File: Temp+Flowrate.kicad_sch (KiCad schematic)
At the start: 24 parts, among them Q1 IRLML0030TRPBF, Q2 IRLML0030TRPBF, U2 TLV9002QDRQ1

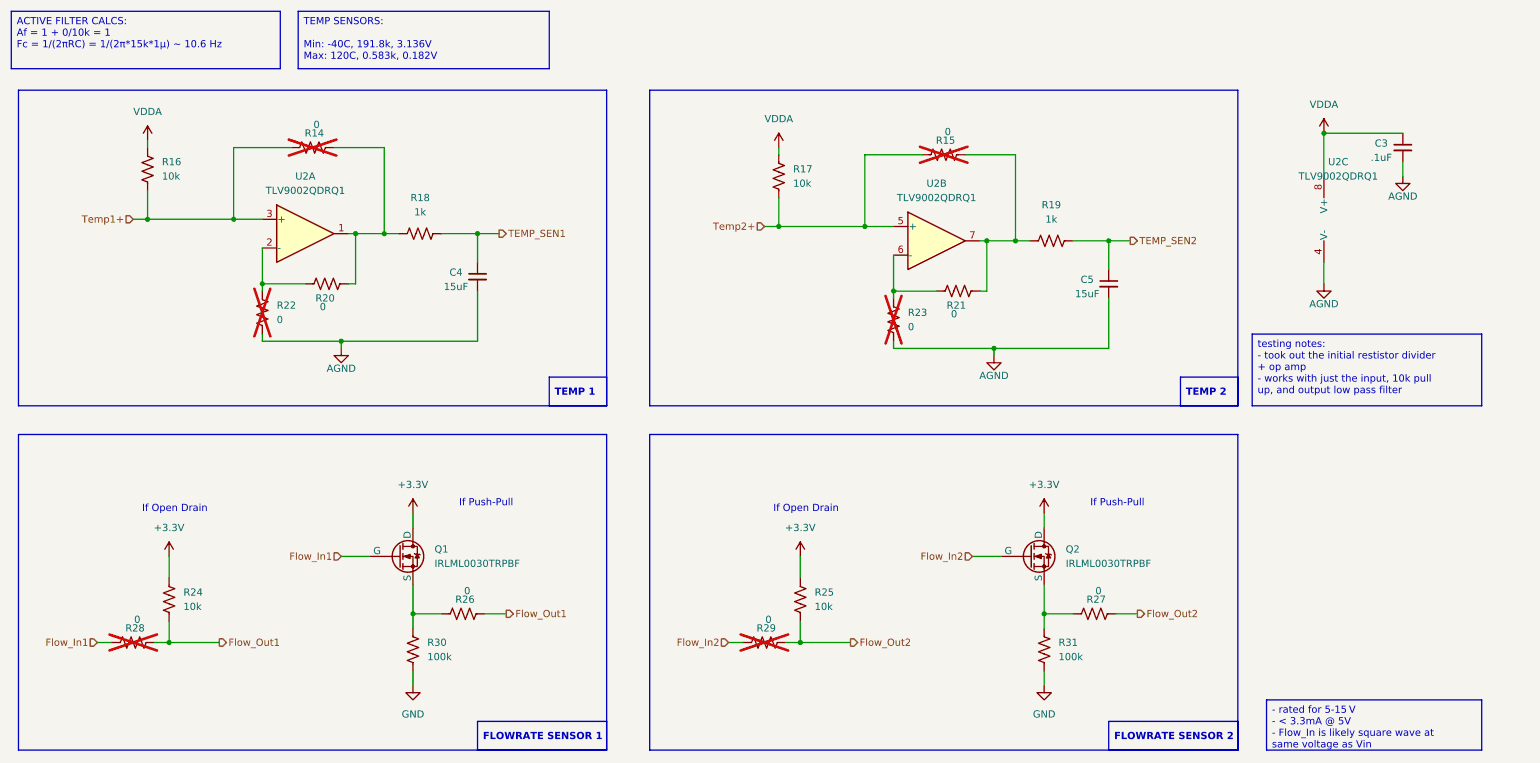
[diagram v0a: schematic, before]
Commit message: lakshays bs
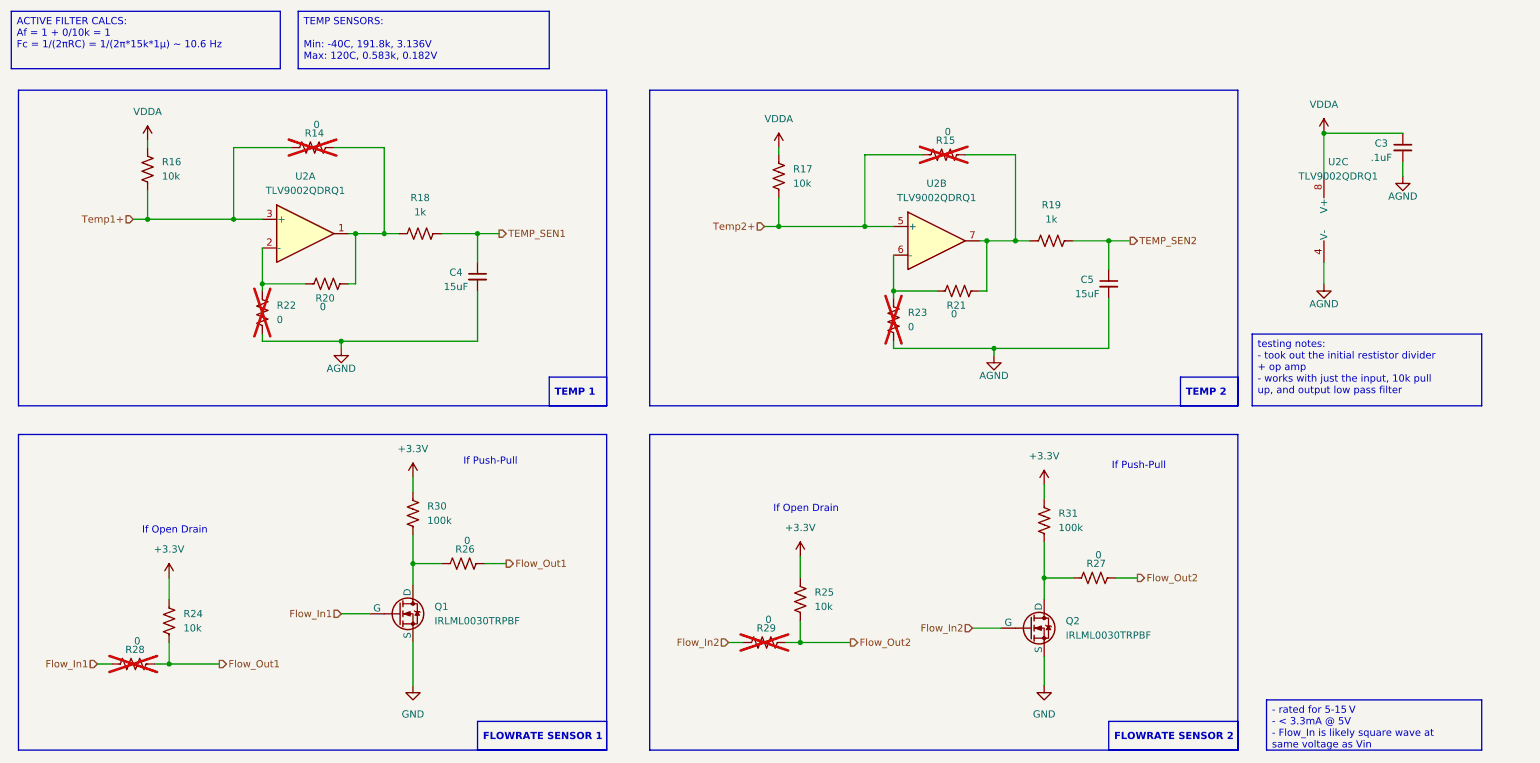
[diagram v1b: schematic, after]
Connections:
- net +3.3V: now also R30.1, R31.1; no longer Q1.3 (D), Q2.3 (D)
- net GND: now also Q1.2 (S), Q2.2 (S); no longer R30.2, R31.2
- new net: Q2.3 (D), R27.1, R31.2
- new net: Q1.3 (D), R26.1, R30.2
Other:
- moved on the sheet: Q1, Q2, R24, R26, R27, R28, R30, R31
